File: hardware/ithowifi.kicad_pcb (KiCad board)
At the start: 2 copper layers, 42.3 x 45.1 mm, 18 parts, among them J1 Conn_02x03_Odd_Even, J2 conn, J3 Conn_Coaxial, Q1 BSS138, Q2 BSS138, U1 WeMos_mini, U2 CC1101-868MHz-Module

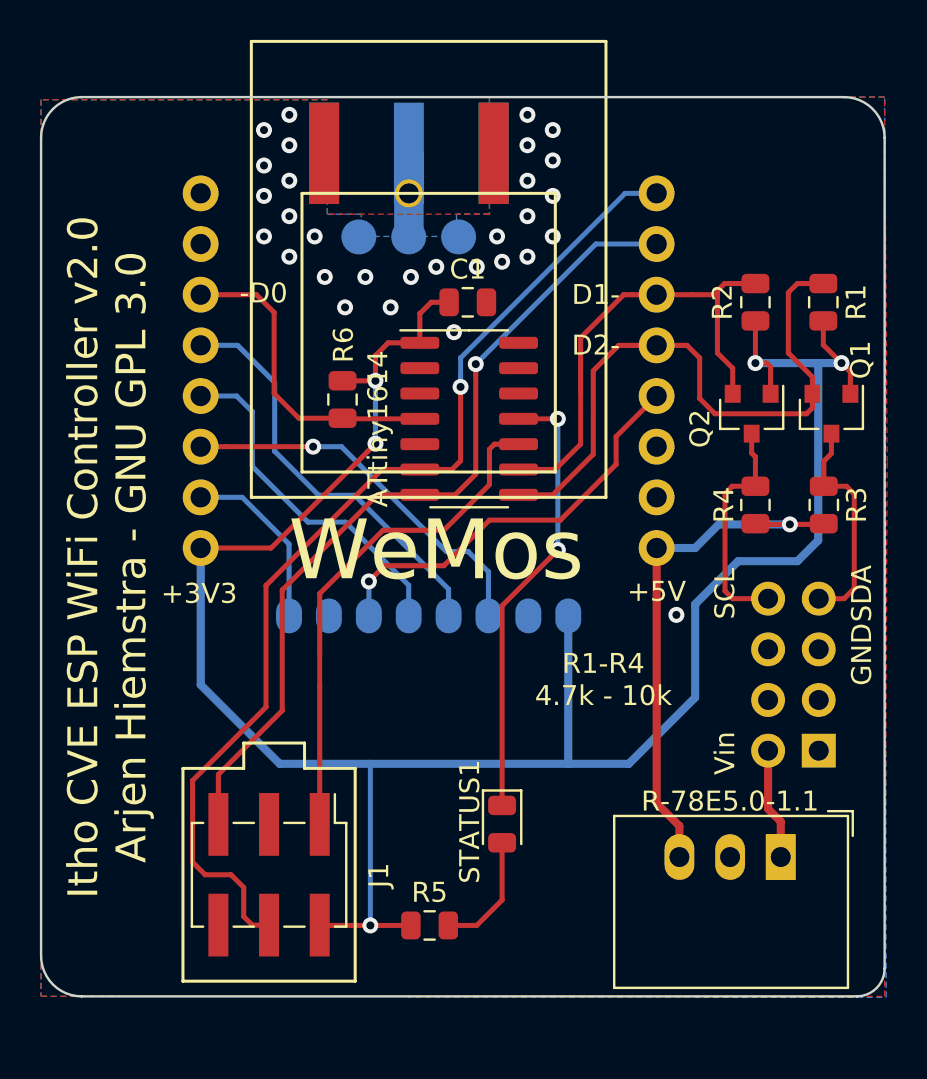
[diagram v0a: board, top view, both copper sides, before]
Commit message: Revert "Test v2.0"
This reverts commit 51a6d60645f7c24e24572af265a76d84da59fee7.
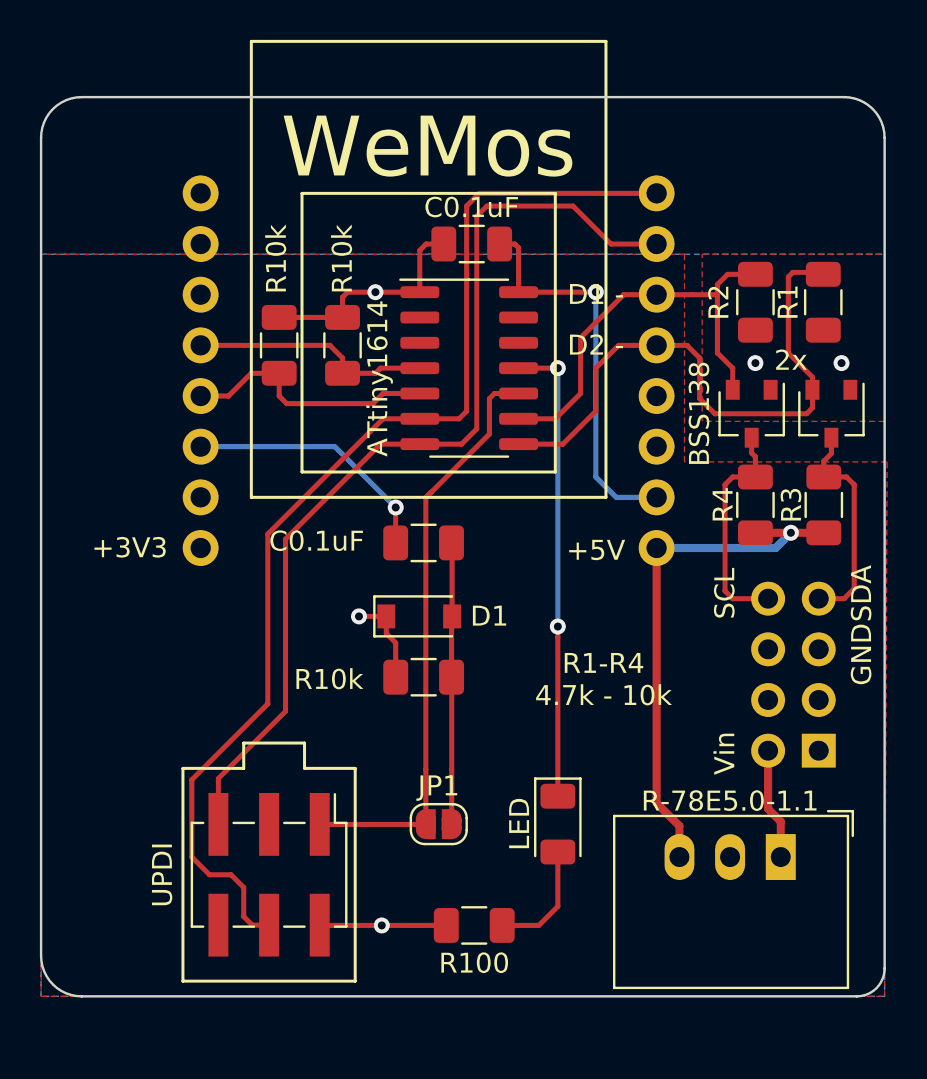
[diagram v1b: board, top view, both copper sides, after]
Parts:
- removed C1: 0,1uF, Inductor_SMD:L_0805_2012Metric
- removed J3: Conn_Coaxial, Connector_Coaxial:SMA_Amphenol_132289_EdgeMount
- removed R6: R10K, Resistor_SMD:R_0805_2012Metric
- removed REF**: MountingHole_2.5mm_Pad, MountingHole:MountingHole_2.5mm_Pad
- removed U2: CC1101-868MHz-Module, nrg_watch:CC1101-868MHz-Module
- added C0.1uF: 0.1uF, Inductor_SMD:L_1206_3216Metric, F.Cu at (104.6, 112.4)
- added C0.1uF: C0.1uF, Inductor_SMD:L_1206_3216Metric, F.Cu at (102.2, 127.4)
- added D1: D, Diode_SMD:D_SOD-123, F.Cu at (102.0, 131.1)
- added JP1: SolderJumper_2_Open, Jumper:SolderJumper-2_P1.3mm_Open_RoundedPad1.0x1.5mm, F.Cu at (103.0, 141.5)
- added R10k: R10K, Resistor_SMD:R_1206_3216Metric, F.Cu at (95.0, 117.5)
- added R10k: R10K, Resistor_SMD:R_1206_3216Metric, F.Cu at (98.2, 117.5)
- added R10k: R10K, Resistor_SMD:R_1206_3216Metric, F.Cu at (102.2, 134.1)
- 2x: renamed from Q1; footprint Package_TO_SOT_SMD:SOT-23 -> Package_TO_SOT_SMD:SOT-23W
- BSS138: renamed from Q2; footprint Package_TO_SOT_SMD:SOT-23 -> Package_TO_SOT_SMD:SOT-23W
- LED: renamed from STATUS1; footprint LED_SMD:LED_0805_2012Metric -> LED_SMD:LED_1206_3216Metric
- R1, R2, R3, R4: footprint Resistor_SMD:R_0805_2012Metric -> Resistor_SMD:R_1206_3216Metric
- R100: renamed from R5; footprint Resistor_SMD:R_0805_2012Metric -> Resistor_SMD:R_1206_3216Metric
- moved LED 2.79 mm to (109.0, 141.5)
- moved ATtiny1614 2.54 mm to (104.5, 118.6)
- moved R100 2.24 mm to (104.8, 146.6)
- renumbered J1 to UPDI
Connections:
- U1 pad 11: Net-(ATtiny1614-Pad4) -> Net-(U1-Pad11)
- U1 pad 12: CLK -> Net-(ATtiny1614-Pad4)
- U1 pad 13: MISO -> Net-(ATtiny1614-Pad5)
- U1 pad 14: MOSI -> Net-(C0.1uF1-Pad1)
- U1 pad 15: CS -> Net-(U1-Pad15)
- U1 pad 4: IRQ -> Net-(U1-Pad4)
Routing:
- net +3V3: track 111.7 -> 22.6 mm
- net CLK: track 20.9 -> 0.00 mm
- net IRQ: track 20.8 -> 0.00 mm, vias 1 -> 0
- net GND: track 0.00 -> 19.9 mm, vias 30 -> 1
- net MOSI: track 19.2 -> 0.00 mm, vias 1 -> 0
- net MISO: track 17.5 -> 0.00 mm
- net Net-(C0.1uF1-Pad2): track 0.00 -> 14.1 mm
- net Net-(ATtiny1614-Pad5): track 0.00 -> 13.0 mm
- net Net-(C0.1uF1-Pad1): track 0.00 -> 12.8 mm, vias 0 -> 1
- net CS: track 9.00 -> 0.00 mm
- net Net-(ATtiny1614-Pad7): track 43.2 -> 48.3 mm, vias 1 -> 0
- net Net-(ATtiny1614-Pad6): track 52.1 -> 56.5 mm, vias 1 -> 0
- net Net-(J3-Pad1): track 4.22 -> 0.00 mm
- net Net-(ATtiny1614-Pad10): track 25.7 -> 29.9 mm
- net Net-(ATtiny1614-Pad4): track 15.9 -> 12.1 mm
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- added copper zone on B.Cu, net +3V3
- added copper zone on F.Cu, net +3V3
- removed copper zone on B.Cu, net GND
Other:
- board text added: "D1 -"
- board text added: "D2 -"
- board text added: "Itho CVE ESP WiFi Controller v1.2 Arjen Hiemstra GNU General Public License 3.0 github.com/arjenhiemstra/ithowifi"
- board text removed: "-D0"
- board text removed: "D1-"
- board text removed: "D2-"
- board text removed: "Itho CVE ESP WiFi Controller v2.0 Arjen Hiemstra - GNU GPL 3.0"
- board text removed: "https://github.com/arjenhiemstra/ithowifi"

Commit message: Test v2.0
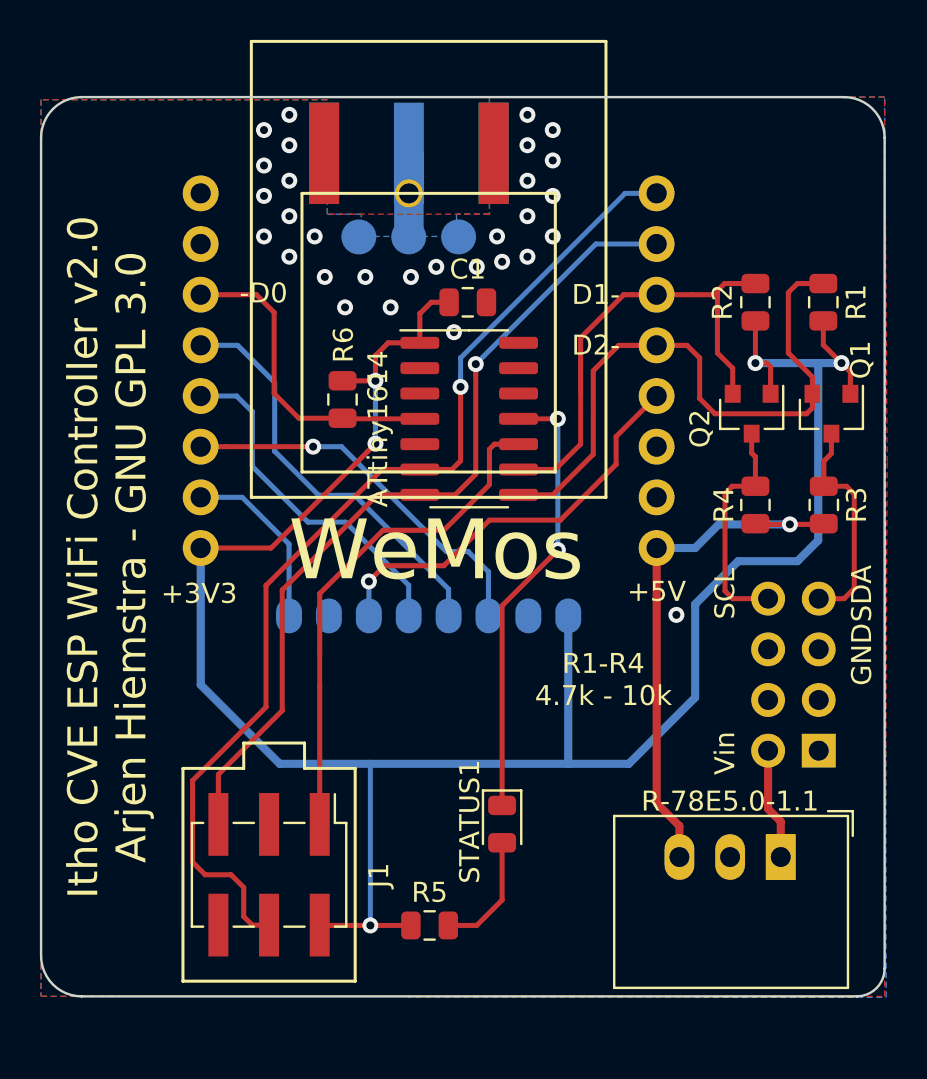
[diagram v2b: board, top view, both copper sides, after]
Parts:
- removed C0.1uF: 0.1uF, Inductor_SMD:L_1206_3216Metric
- removed C0.1uF: C0.1uF, Inductor_SMD:L_1206_3216Metric
- removed D1: D, Diode_SMD:D_SOD-123
- removed JP1: SolderJumper_2_Open, Jumper:SolderJumper-2_P1.3mm_Open_RoundedPad1.0x1.5mm
- removed R10k (x3): R10K, Resistor_SMD:R_1206_3216Metric
- added C1: 0,1uF, Inductor_SMD:L_0805_2012Metric, F.Cu at (104.5, 115.3)
- added J3: Conn_Coaxial, Connector_Coaxial:SMA_Amphenol_132289_EdgeMount, B.Cu at (101.5, 107.8)
- added R6: R10K, Resistor_SMD:R_0805_2012Metric, F.Cu at (98.2, 120.2)
- added REF**: MountingHole_2.5mm_Pad, MountingHole:MountingHole_2.5mm_Pad, F.Cu at (101.5, 109.9)
- added U2: CC1101-868MHz-Module, nrg_watch:CC1101-868MHz-Module, B.Cu at (102.5, 121.5)
- Q1: renamed from 2x; footprint Package_TO_SOT_SMD:SOT-23W -> Package_TO_SOT_SMD:SOT-23
- Q2: renamed from BSS138; footprint Package_TO_SOT_SMD:SOT-23W -> Package_TO_SOT_SMD:SOT-23
- R1, R2, R3, R4: footprint Resistor_SMD:R_1206_3216Metric -> Resistor_SMD:R_0805_2012Metric
- R5: renamed from R100; footprint Resistor_SMD:R_1206_3216Metric -> Resistor_SMD:R_0805_2012Metric
- STATUS1: renamed from LED; footprint LED_SMD:LED_1206_3216Metric -> LED_SMD:LED_0805_2012Metric
- moved STATUS1 2.79 mm to (106.2, 141.5)
- moved ATtiny1614 2.54 mm to (104.5, 121.2)
- moved R5 2.24 mm to (102.5, 146.6)
- renumbered UPDI to J1
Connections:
- U1 pad 11: Net-(U1-Pad11) -> Net-(ATtiny1614-Pad4)
- U1 pad 12: Net-(ATtiny1614-Pad4) -> CLK
- U1 pad 13: Net-(ATtiny1614-Pad5) -> MISO
- U1 pad 14: Net-(C0.1uF1-Pad1) -> MOSI
- U1 pad 15: Net-(U1-Pad15) -> CS
- U1 pad 4: Net-(U1-Pad4) -> IRQ
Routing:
- net +3V3: track 22.6 -> 111.7 mm
- net CLK: track 0.00 -> 20.9 mm
- net IRQ: track 0.00 -> 20.8 mm, vias 0 -> 1
- net GND: track 19.9 -> 0.00 mm, vias 1 -> 30
- net MOSI: track 0.00 -> 19.2 mm, vias 0 -> 1
- net MISO: track 0.00 -> 17.5 mm
- net Net-(C0.1uF1-Pad2): track 14.1 -> 0.00 mm
- net Net-(ATtiny1614-Pad5): track 13.0 -> 0.00 mm
- net Net-(C0.1uF1-Pad1): track 12.8 -> 0.00 mm, vias 1 -> 0
- net CS: track 0.00 -> 9.00 mm
- net Net-(ATtiny1614-Pad7): track 48.3 -> 43.2 mm, vias 0 -> 1
- net Net-(ATtiny1614-Pad6): track 56.5 -> 52.1 mm, vias 0 -> 1
- net Net-(J3-Pad1): track 0.00 -> 4.22 mm
- net Net-(ATtiny1614-Pad10): track 29.9 -> 25.7 mm
- net Net-(ATtiny1614-Pad4): track 12.1 -> 15.9 mm
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- added copper zone on B.Cu, net GND
- removed copper zone on B.Cu, net +3V3
- removed copper zone on F.Cu, net +3V3
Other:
- board text added: "-D0"
- board text added: "D1-"
- board text added: "D2-"
- board text added: "Itho CVE ESP WiFi Controller v2.0 Arjen Hiemstra - GNU GPL 3.0"
- board text added: "https://github.com/arjenhiemstra/ithowifi"
- board text removed: "D1 -"
- board text removed: "D2 -"
- board text removed: "Itho CVE ESP WiFi Controller v1.2 Arjen Hiemstra GNU General Public License 3.0 github.com/arjenhiemstra/ithowifi"
